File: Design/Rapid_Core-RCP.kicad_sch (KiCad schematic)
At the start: 77 parts, among them IC1 TLIN1039DDFRQ1, IC2 TLIN1039DDFRQ1, IC3 SHT30A-DIS-B2.5KS, J1 LIN-2, J2 LIN-1, J3 LIN-1, J4 LIN-2, J5 GPIO_CONN_X_4, J6 SWD_Debug, J7 SPI, J8 USART, SW1 SW_Push, U1 STM32F446RETx, Y1 Crystal_GND24, Y2 32.768_KHz

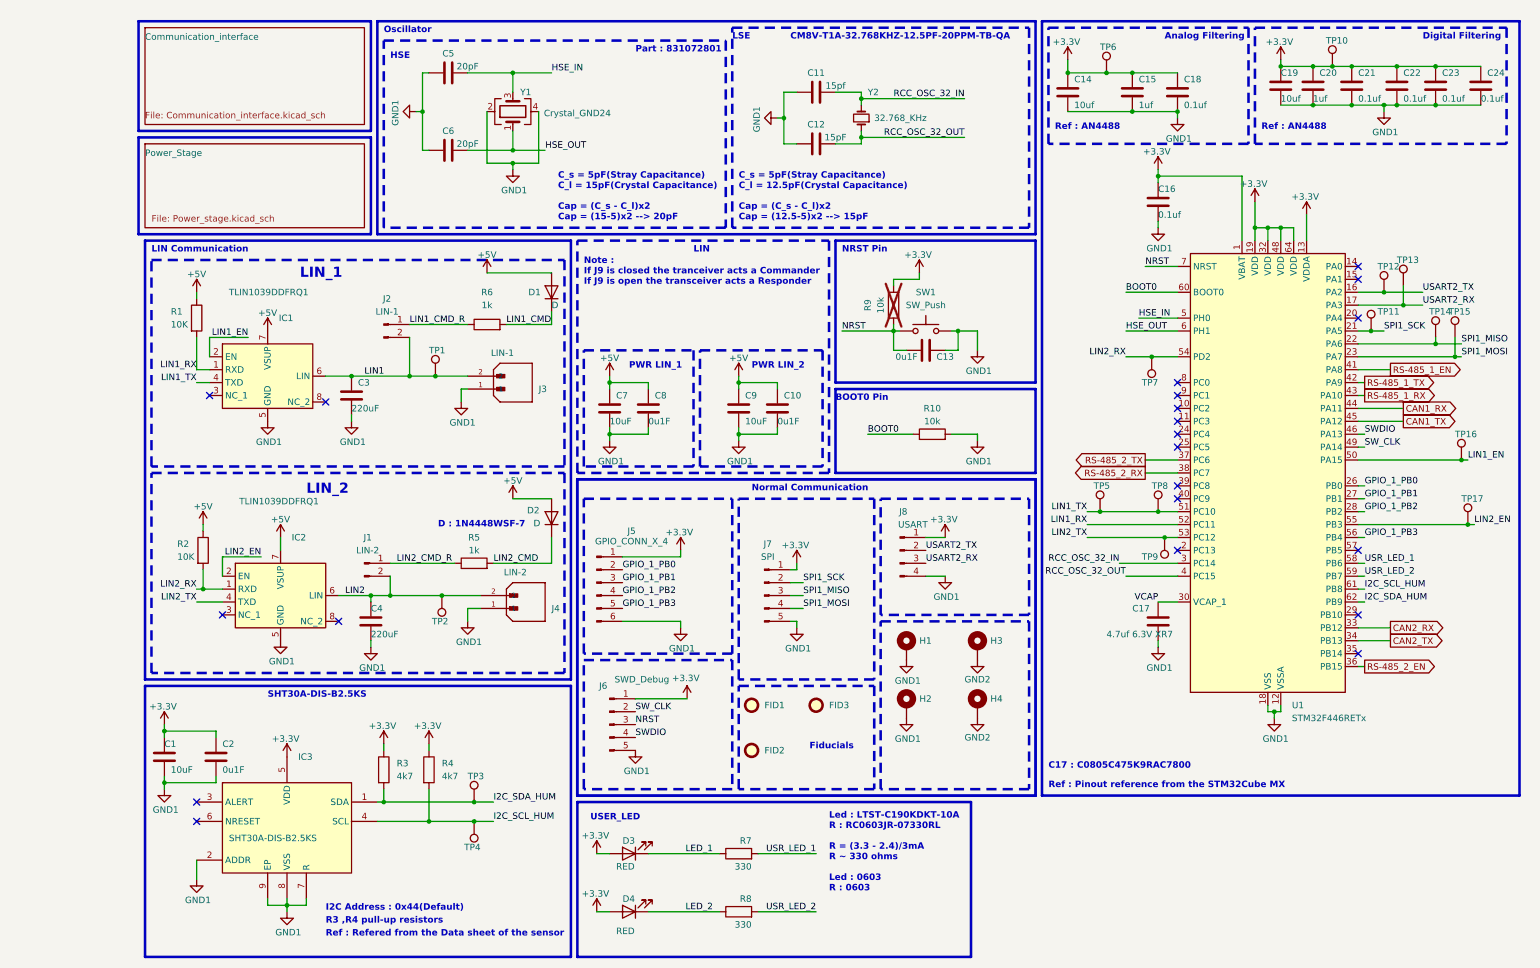
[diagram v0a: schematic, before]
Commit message: Added Information to all the sheets
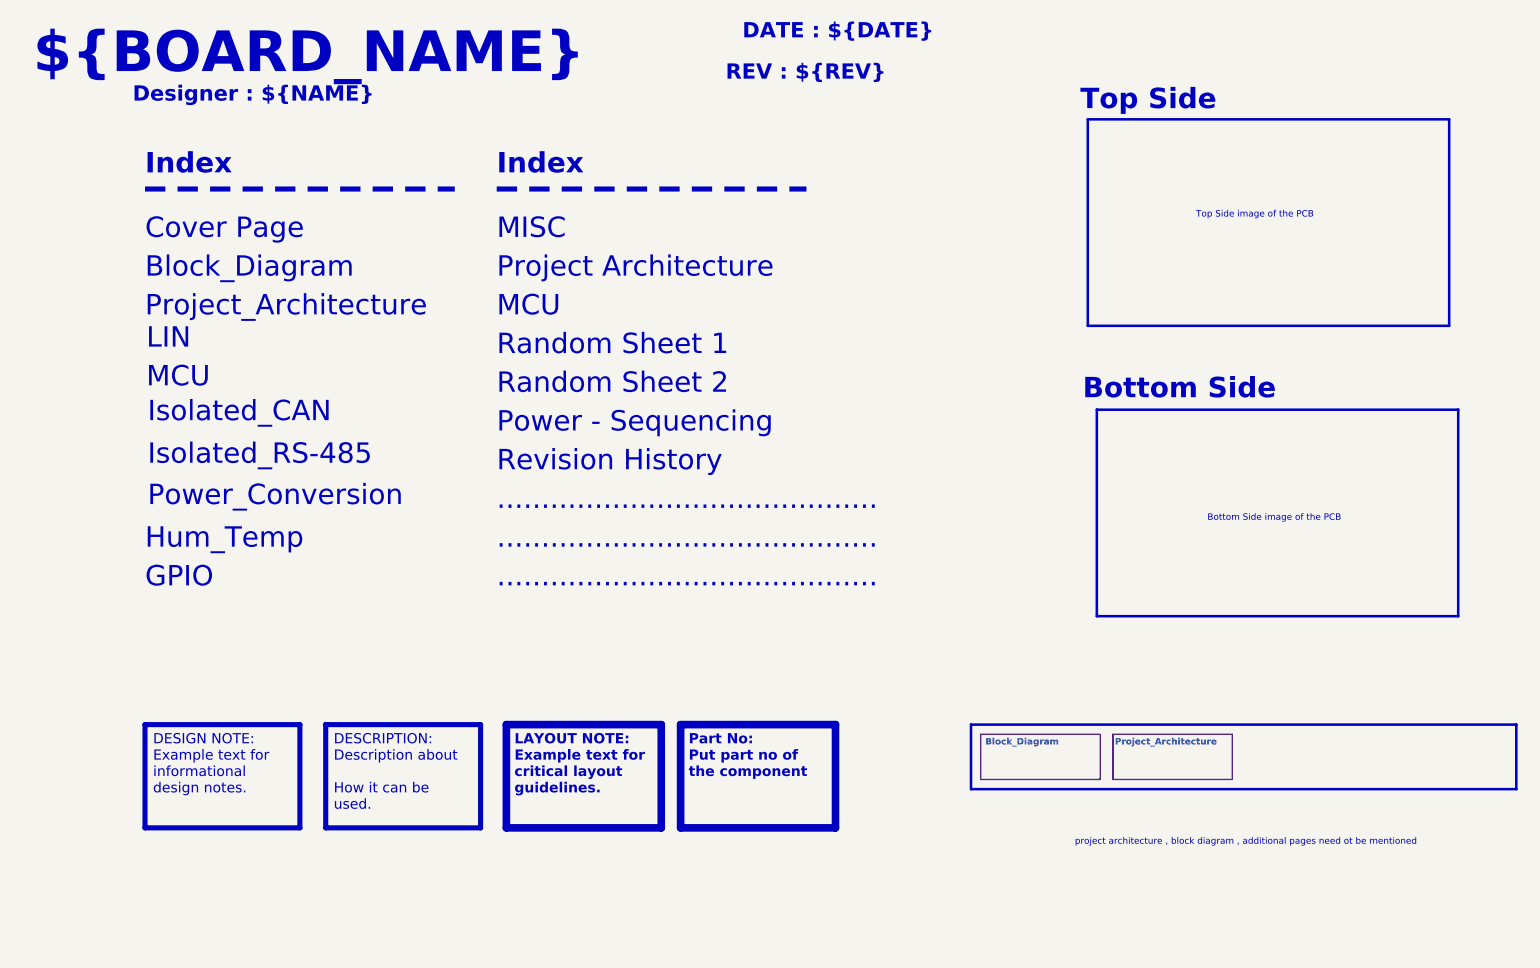
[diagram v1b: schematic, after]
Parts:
- removed C1, C7, C9: 10uF, Capacitor_SMD:C_0805_2012Metric_Pad1.18x1.45mm_HandSolder, symbol Device:C
- removed C10, C13, C2, C8: 0u1F, Capacitor_SMD:C_0603_1608Metric_Pad1.08x0.95mm_HandSolder, symbol Device:C
- removed C11: 15pf, Capacitor_SMD:C_0603_1608Metric, symbol Device:C
- removed C12: 15pF, Capacitor_SMD:C_0603_1608Metric, symbol Device:C
- removed C14, C19: 10uf, Capacitor_SMD:C_0805_2012Metric_Pad1.18x1.45mm_HandSolder, symbol Device:C
- removed C15, C20: 1uf, Capacitor_SMD:C_0603_1608Metric_Pad1.08x0.95mm_HandSolder, symbol Device:C
- removed C16, C18, C21, C22, C23, C24: 0.1uf, Capacitor_SMD:C_0603_1608Metric_Pad1.08x0.95mm_HandSolder, symbol Device:C
- removed C17: 4.7uf 6.3V XR7, Capacitor_SMD:C_0805_2012Metric_Pad1.18x1.45mm_HandSolder, symbol Device:C
- removed C3, C4: 220uF, Capacitor_SMD:C_0805_2012Metric_Pad1.18x1.45mm_HandSolder, symbol Device:C
- removed C5, C6: 20pF, Capacitor_SMD:C_0603_1608Metric, symbol Device:C
- removed D1, D2: D, Diode_SMD:D_SOD-323_HandSoldering, symbol Device:D
- removed D3, D4: RED, LED_SMD:LED_0603_1608Metric_Pad1.05x0.95mm_HandSolder, symbol Device:LED
- removed FID1, FID2, FID3: Fiducial, Fiducial:Fiducial_1.5mm_Mask3mm, symbol Mechanical:Fiducial
- removed H1, H2, H3, H4: MountingHole_Pad, MountingHole:MountingHole_2.2mm_M2_Pad, symbol Mechanical:MountingHole_Pad
- removed IC1, IC2: TLIN1039DDFRQ1, TLIN1039DDFRQ1:SOT65P280X110-8N, symbol TLIN1039DDFRQ1:TLIN1039DDFRQ1
- removed IC3: SHT30A-DIS-B2.5KS, SHT30A-DIS-B2.5KS:SON50P250X250X100-9N-D, symbol SHT30A-DIS-B2_5KS:SHT30A-DIS-B2.5KS
- removed J1: LIN-2, Connector_PinHeader_2.54mm:PinHeader_1x02_P2.54mm_Vertical, symbol Connector:Conn_01x02_Pin
- removed J2: LIN-1, Connector_PinHeader_2.54mm:PinHeader_1x02_P2.54mm_Vertical, symbol Connector:Conn_01x02_Pin
- removed J3: LIN-1, 0530480210_2pin_P1.25_PicoBlade:MOLEX_530480210, symbol 0530480210_2pin_P1.25_PicoBlade:530480210
- removed J4: LIN-2, 0530480210_2pin_P1.25_PicoBlade:MOLEX_530480210, symbol 0530480210_2pin_P1.25_PicoBlade:530480210
- removed J5: GPIO_CONN_X_4, Connector_PinHeader_2.54mm:PinHeader_1x06_P2.54mm_Vertical, symbol Connector:Conn_01x06_Pin
- removed J6: SWD_Debug, Connector_PinHeader_2.54mm:PinHeader_1x05_P2.54mm_Vertical, symbol Connector:Conn_01x05_Pin
- removed J7: SPI, Connector_PinHeader_2.54mm:PinHeader_1x05_P2.54mm_Vertical, symbol Connector:Conn_01x05_Pin
- removed J8: USART, Connector_PinHeader_2.54mm:PinHeader_1x04_P2.54mm_Vertical, symbol Connector:Conn_01x04_Pin
- removed R1, R2: 10K, Resistor_SMD:R_0805_2012Metric_Pad1.20x1.40mm_HandSolder, symbol Device:R
- removed R10, R9: 10k, Resistor_SMD:R_0805_2012Metric_Pad1.20x1.40mm_HandSolder, symbol Device:R
- removed R3, R4: 4k7, Resistor_SMD:R_0805_2012Metric_Pad1.20x1.40mm_HandSolder, symbol Device:R
- removed R5, R6: 1k, Resistor_SMD:R_0805_2012Metric_Pad1.20x1.40mm_HandSolder, symbol Device:R
- removed R7, R8: 330, Resistor_SMD:R_0603_1608Metric_Pad0.98x0.95mm_HandSolder, symbol Device:R
- removed SW1: SW_Push, Button_Switch_SMD:SW_Tactile_SPST_NO_Straight_CK_PTS636Sx25SMTRLFS, symbol Switch:SW_Push
- removed TP1, TP10, TP11, TP12, TP13, TP14, TP15, TP16, TP17, TP2, TP3, TP4, TP5, TP6, TP7, TP8, TP9: TestPoint, TestPoint:TestPoint_Pad_D1.0mm, symbol Connector:TestPoint
- removed U1: STM32F446RETx, Package_QFP:LQFP-64_10x10mm_P0.5mm, symbol MCU_ST_STM32F4:STM32F446RETx
- removed Y1: Crystal_GND24, Crystal:Crystal_SMD_2520-4Pin_2.5x2.0mm, symbol Device:Crystal_GND24
- removed Y2: 32.768_KHz, Crystal:Crystal_SMD_MicroCrystal_CC8V-T1A-2Pin_2.0x1.2mm, symbol Device:Crystal_Small
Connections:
- no-connect marks 21 -> 0
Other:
- removed sheet Communication_interface
- removed sheet Power_Stage
- added sheet Block_Diagram (Block_Diagram.kicad_sch)
- added sheet Project_Architecture (Project_Architecture.kicad_sch)
- note added: "${BOARD_NAME}"
- note added: "..........................................."
- note added: "Block_Diagram"
- note added: "Bottom Side"
- note added: "Bottom Side image of the PCB"
- note added: "Cover Page"
- note added: "DATE : ${DATE}"
- note added: "Designer : ${NAME}"
- note added: "GPIO"
- note added: "Hum_Temp"
- note added: "Index"
- note added: "Isolated_CAN"
- note added: "Isolated_RS-485"
- note added: "MCU"
- note added: "MISC"
- note added: "Power - Sequencing"
- note added: "Power_Conversion"
- note added: "Project Architecture"
- note added: "Project_Architecture"
- note added: "REV : ${REV}"
- note added: "Random Sheet 1"
- note added: "Random Sheet 2"
- note added: "Revision History"
- note added: "Top Side"
- note added: "Top Side image of the PCB"
- note added: "project architecture , block diagram , additional pages need ot be mentioned"
- note removed: "Analog Filtering"
- note removed: "BOOT0 Pin"
- note removed: "C17 : C0805C475K9RAC7800"
- note removed: "CM8V-T1A-32.768KHZ-12.5PF-20PPM-TB-QA"
- note removed: "C_s = 5pF(Stray Capacitance) C_l = 12.5pF(Crystal Capacitance) Cap = (C_s - C_l)x2 Cap = (12.5-5)x2 --> 15pF"
- note removed: "C_s = 5pF(Stray Capacitance) C_l = 15pF(Crystal Capacitance) Cap = (C_s - C_l)x2 Cap = (15-5)x2 --> 20pF"
- note removed: "D : 1N4448WSF-7"
- note removed: "Digital Filtering"
- note removed: "Fiducials"
- note removed: "HSE"
- note removed: "I2C Address : 0x44(Default)"
- note removed: "LIN Communication"
- note removed: "LIN_1"
- note removed: "LIN_2"
- note removed: "LSE"
- note removed: "Led : LTST-C190KDKT-10A R : RC0603JR-07330RL R = (3.3 - 2.4)/3mA R ~ 330 ohms Led : 0603 R : 0603"
- note removed: "NRST Pin"
- note removed: "Normal Communication"
- note removed: "Note : If J9 is closed the tranceiver acts a Commander If J9 is open the transceiver acts a Responder"
- note removed: "Oscillator"
- note removed: "PWR LIN_1"
- note removed: "PWR LIN_2"
- note removed: "Part : 831072801"
- note removed: "R3 ,R4 pull-up resistors"
- note removed: "Ref : AN4488"
- note removed: "Ref : Pinout reference from the STM32Cube MX"
- note removed: "Ref : Refered from the Data sheet of the sensor"
- note removed: "SHT30A-DIS-B2.5KS"
- note removed: "USER_LED"
